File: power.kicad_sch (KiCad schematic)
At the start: 21 parts, among them J1 USB_C_Receptacle_USB2.0_16P, U40 RP2040, U41 W25Q128JVS, U42 MIC5219-3.3YM5, Y1 12MHz

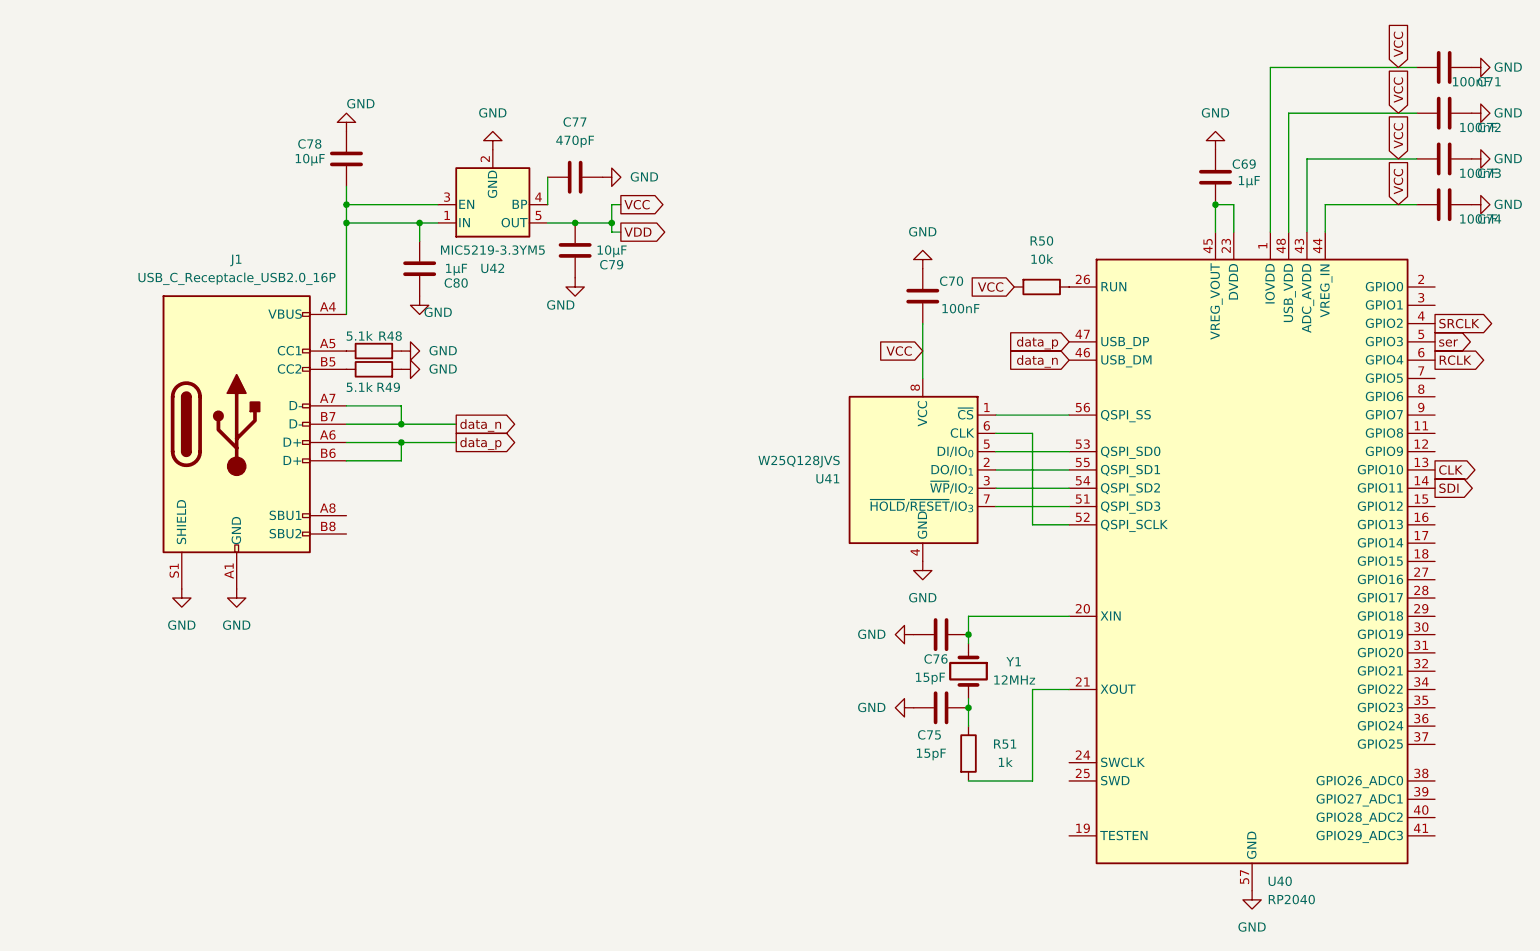
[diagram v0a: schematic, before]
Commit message: Updated: pots
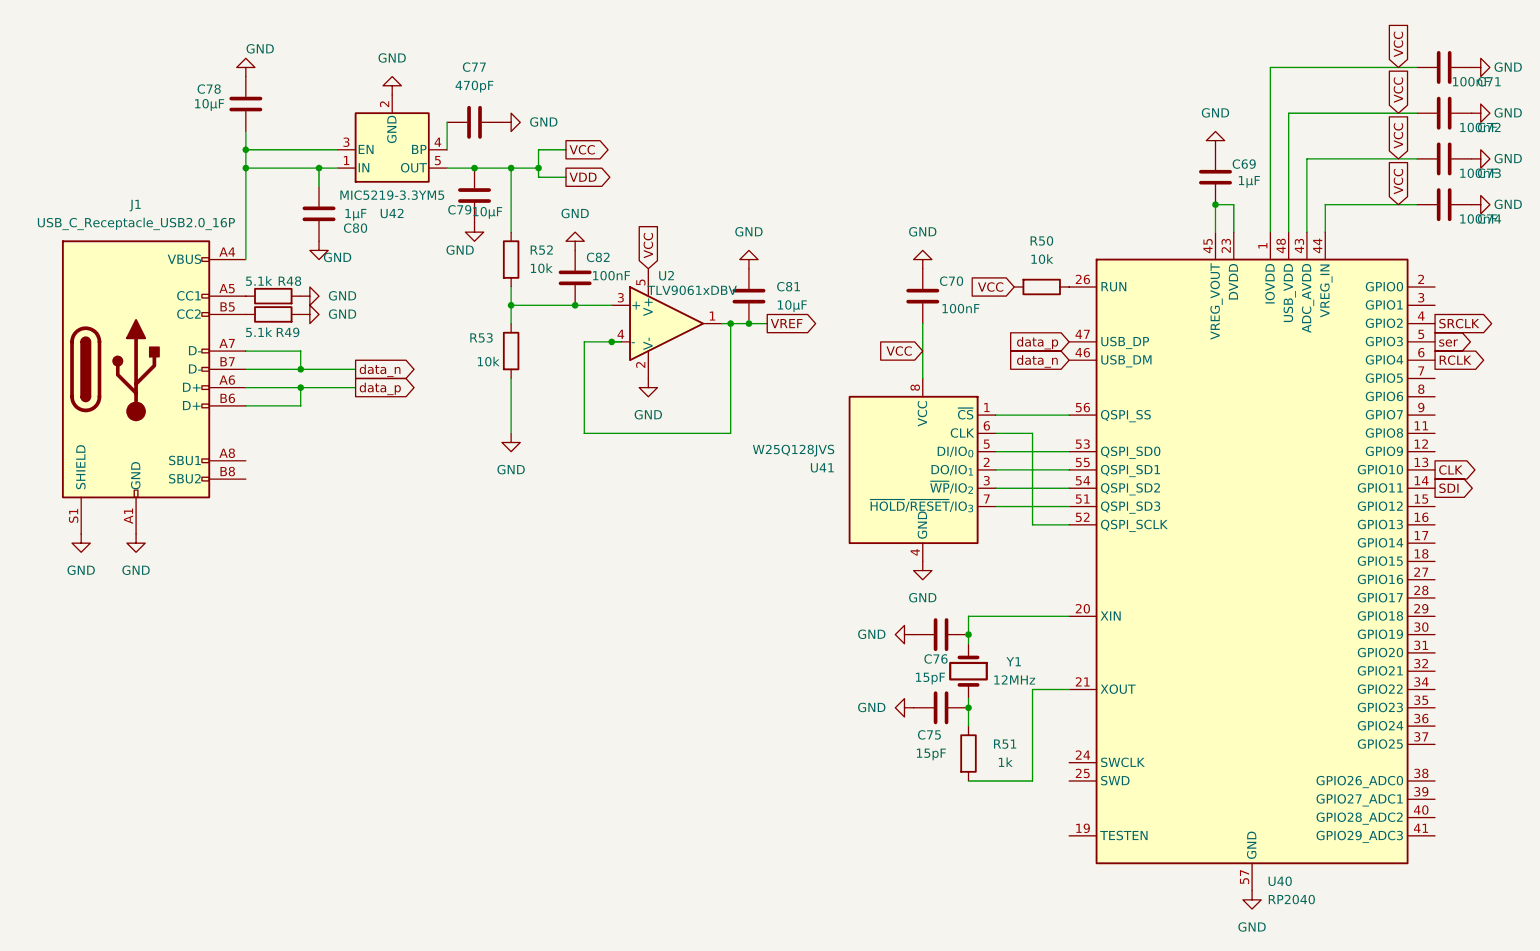
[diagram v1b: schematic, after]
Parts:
- added C81: 10µF, symbol Device:C
- added C82: 100nF, symbol Device:C
- added R52, R53: 10k, symbol Device:R
- added U2: TLV9061xDBV, Package_TO_SOT_SMD:SOT-23-5, symbol Amplifier_Operational:TLV9061xDBV
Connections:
- net GND: now also C81.1, C82.1, R53.2, U2.2 (V-)
- net VCC: now also R52.1, U2.5 (V+)
- new net: C82.2, R52.2, R53.1, U2.3 (+)
- new net VREF: C81.2, U2.1, U2.4 (-)
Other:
- moved on the sheet: C77, C78, C79, C80, J1, R48, R49, U42
